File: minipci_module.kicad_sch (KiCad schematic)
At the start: 7 parts, among them CON3 2041119-1, U17 IP4220CZ6, U18 IP4220CZ6

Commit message: Gerbers created, BOM, CPL
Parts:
- removed R73, R74: 4k7, Resistor_Smd_0402:4k7_0402, symbol Resistors_Smd0402:4k7
- removed R75, R76: 1k, Resistor_Smd_0402:1k_0402, symbol Resistors_Smd0402:1k
- added R73, R74: 4k7, Resistor_Smd_0603:4k7_0603, symbol Resistors_Smd0603:4k7
- added R75, R76: 1k, Resistor_Smd_0603:1k_0603, symbol Resistors_Smd0603:1k
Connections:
- net 3V3: now also R73.1, R74.1
- net GND: now also R75.2, R76.2
- net GPS_PPS/UART_TX: now also R76.1
- net SCL: now also R73.2
- net SDA: now also R74.2
- net SPDT_SEL-~{WDISABLE}/UART_RX: now also R75.1

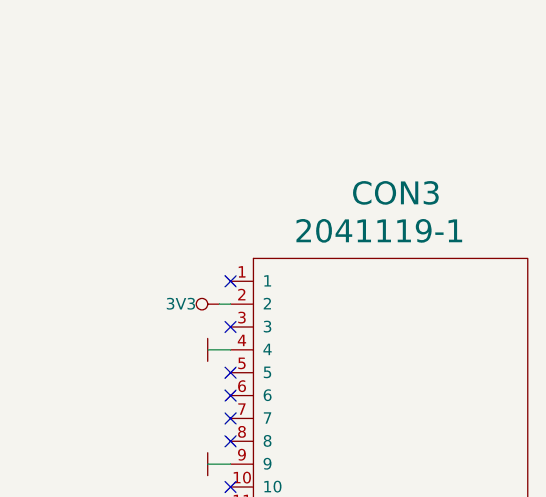
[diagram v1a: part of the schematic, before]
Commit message: New branch created
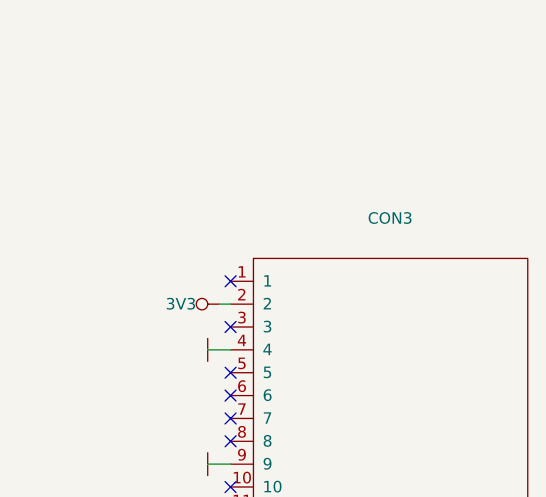
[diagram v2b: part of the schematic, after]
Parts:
- removed CON3: 2041119-1, Smd_Connectors:2041119-1, symbol Smd_Connectors:2041119-1
- added CON3: (no value), symbol Smd_Connectors:119A-80A00-R02-SET
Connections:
- net 3V3: now also CON3.2, CON3.24, CON3.39, CON3.41, CON3.52
- net GND: now also CON3.0 (PADS), CON3.15, CON3.21, CON3.26, CON3.27, CON3.29, CON3.34, CON3.35, CON3.37, CON3.4, CON3.40, CON3.43, CON3.50, CON3.9
- net GPS_PPS/UART_TX: now also CON3.19
- net SCL: now also CON3.30
- net SDA: now also CON3.32
- net SPDT_SEL-~{WDISABLE}/UART_RX: now also CON3.17
- net SPI_GSN: now also CON3.51
- net SPI_MISO: now also CON3.47
- net SPI_MOSI: now also CON3.49
- net SPI_SCK: now also CON3.45
- net ~{RESET}: now also CON3.22
